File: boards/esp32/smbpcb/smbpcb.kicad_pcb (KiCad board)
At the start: 2 copper layers, 77.7 x 65.3 mm, 57 parts, among them IC1 MiCS-6814, J1 USB_B_Micro, J2 PMS7003, Q1 SUD08P06-155L, Q2 SS8050_NPN, Q3 SS8050_NPN, U1 MCP73831-2-OT, U2 TPS61200DRC, U3 ESP32-WROOM-32, U4 SSD1306, U5 BME680, U6 MH-Z19B

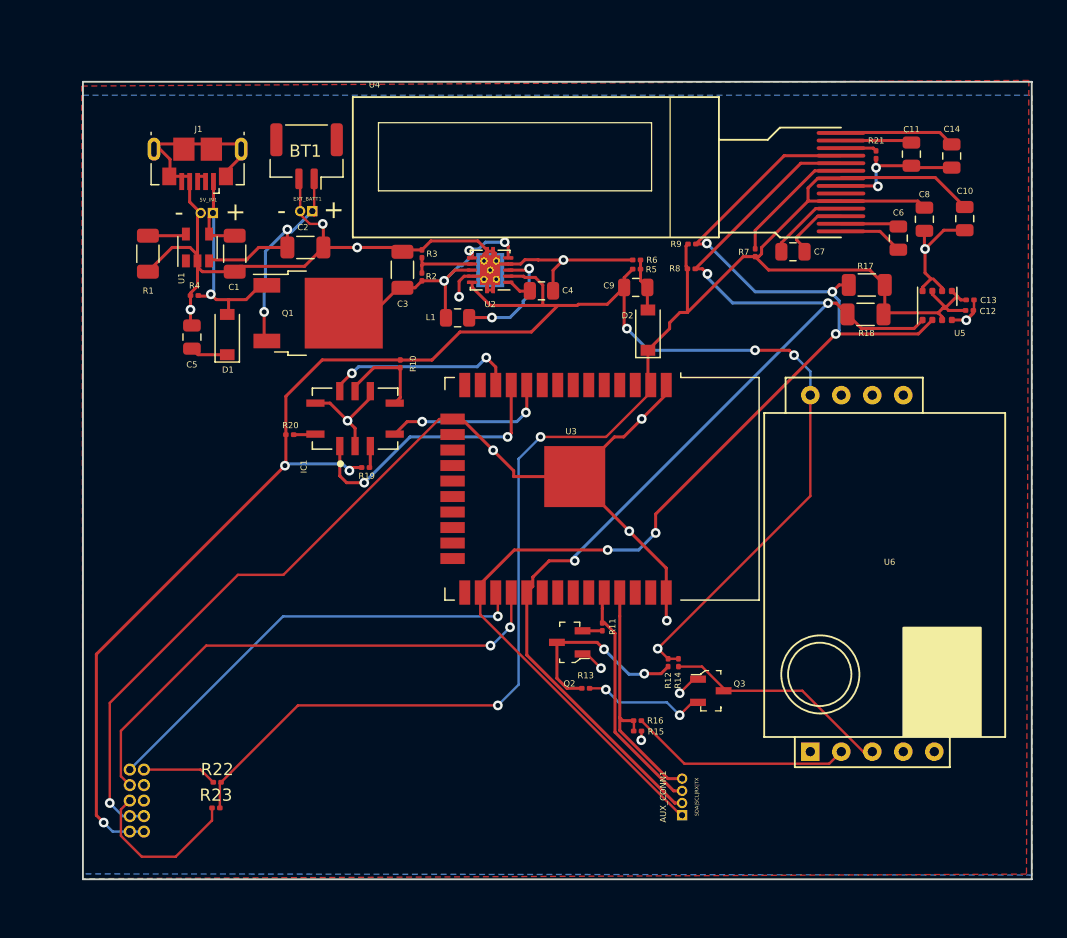
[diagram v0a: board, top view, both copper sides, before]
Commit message: more work'
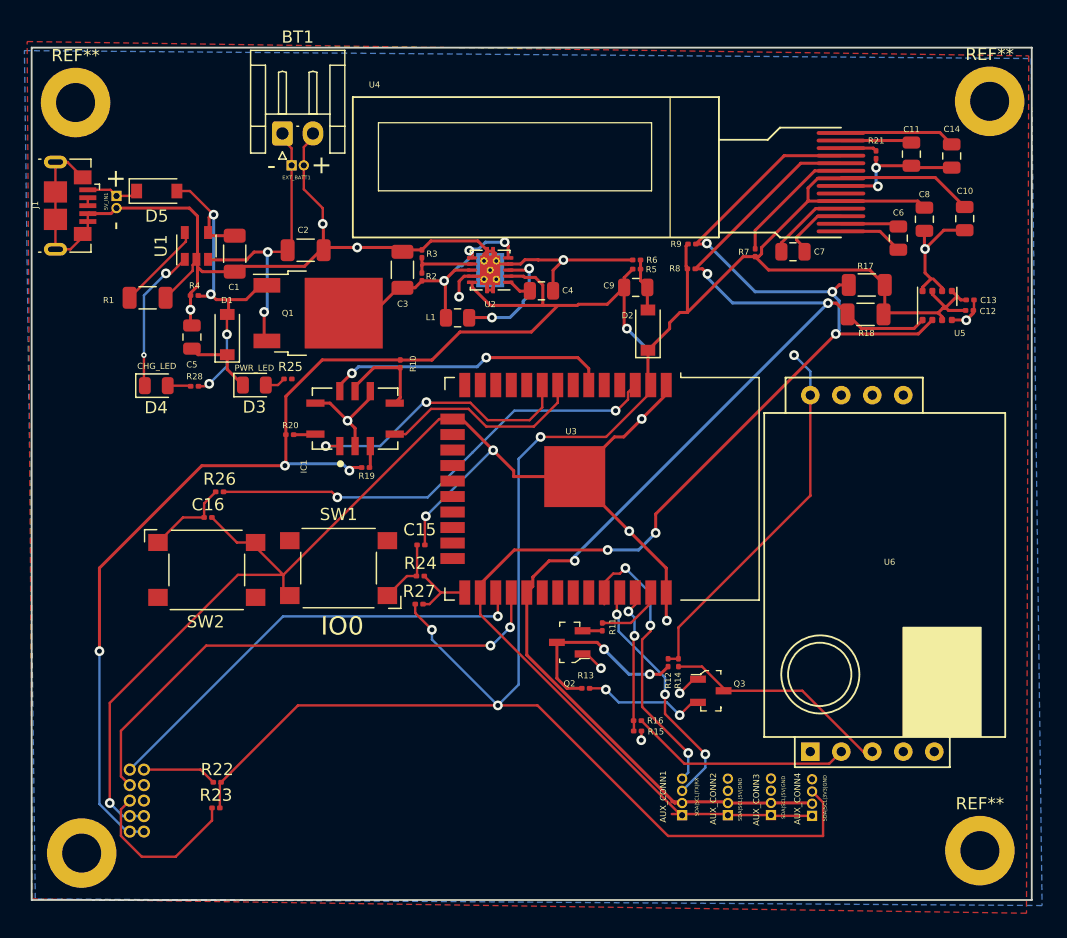
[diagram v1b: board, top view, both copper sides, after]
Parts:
- added ?: , , F.Cu at (74.1, 78.1)
- added AUX_CONN2: Conn_01x04_Female, Connector_PinHeader_1.00mm:PinHeader_1x04_P1.00mm_Vertical, F.Cu at (127.0, 75.0)
- added AUX_CONN3: Conn_01x04_Female, Connector_PinHeader_1.00mm:PinHeader_1x04_P1.00mm_Vertical, F.Cu at (130.6, 75.0)
- added AUX_CONN4: Conn_01x04_Female, Connector_PinHeader_1.00mm:PinHeader_1x04_P1.00mm_Vertical, F.Cu at (133.9, 75.0)
- added C15: 1nF, Capacitor_SMD:C_0201_0603Metric, F.Cu at (101.9, 52.9)
- added C16: 1nF, Capacitor_SMD:C_0201_0603Metric, F.Cu at (84.5, 50.6)
- added D3: PWR_LED, LED_SMD:LED_0805_2012Metric, F.Cu at (88.2, 39.8)
- added D4: PWR_LED, LED_SMD:LED_0805_2012Metric, F.Cu at (80.2, 39.8)
- added D5: D_Schottky, Diode_SMD:D_SOD-123, F.Cu at (80.2, 23.9)
- added R24: 470, Capacitor_SMD:C_0201_0603Metric, F.Cu at (101.8, 55.4)
- added R25: 2k, Capacitor_SMD:C_0201_0603Metric, F.Cu at (91.0, 39.2)
- added R26: 470, Capacitor_SMD:C_0201_0603Metric, F.Cu at (85.4, 48.5)
- added R27: 5.1k, Capacitor_SMD:C_0201_0603Metric, F.Cu at (101.8, 57.7)
- added R28: 470, Capacitor_SMD:C_0201_0603Metric, F.Cu at (83.3, 39.9)
- added REF**: MountingHole_3.2mm_M3_ISO7380_Pad, mountingholes:MountingHole_3.2mm_M3_ISO7380_Pad, F.Cu at (148.5, 16.5)
- added REF**: MountingHole_3.2mm_M3_ISO7380_Pad, mountingholes:MountingHole_3.2mm_M3_ISO7380_Pad, F.Cu at (147.7, 77.9)
- added REF**: MountingHole_3.2mm_M3_ISO7380_Pad, mountingholes:MountingHole_3.2mm_M3_ISO7380_Pad, F.Cu at (73.6, 16.6)
- added SW1: RESET, Button_Switch_SMD:SW_SPST_Omron_B3FS-101xP, F.Cu at (95.2, 54.8)
- added SW2: RESET, Button_Switch_SMD:SW_SPST_Omron_B3FS-101xP, F.Cu at (84.3, 54.9)
- BT1: footprint Connector_JST:JST_GH_SM02B-GHS-TB_1x02-1MP_P1.25mm_Horizontal -> Connector_JST:JST_EH_S2B-EH_1x02_P2.50mm_Horizontal
- R1: value 10k -> 2k
- moved J1 11.0 mm to (73.2, 25.1), turned to -90 degrees
- moved 5V_IN1 8.02 mm to (77.0, 24.2), turned to 0 degrees
- moved EXT_BATT1 4.12 mm to (91.3, 21.8), turned to 90 degrees
- moved R1 3.62 mm to (79.5, 32.6), turned to 0 degrees
- moved BT1 2.72 mm to (90.5, 19.1), turned to 0 degrees
- moved C2 0.22 mm to (92.5, 28.7)
- moved U1 0.15 mm to (83.5, 28.4)
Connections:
- AUX_CONN1 pad 3: ESP_RX0 -> ESP_TX0
- AUX_CONN1 pad 4: ESP_TX0 -> ESP_RX0
- C1 pad 1: Net-(5V_IN1-Pad1) -> Net-(C1-Pad1)
- D1 pad 2: Net-(5V_IN1-Pad1) -> Net-(C1-Pad1)
- J2 pad 7: ESP_RX1 -> ESP_RX2
- J2 pad 9: ESP_TX1 -> ESP_TX2
- Q1 pad 1: Net-(5V_IN1-Pad1) -> Net-(C1-Pad1)
- R11 pad 1: ESP_RX0 -> ESP_RX1
- R15 pad 2: ESP_TX0 -> ESP_TX1
- R16 pad 1: ESP_TX0 -> ESP_TX1
- R4 pad 1: Net-(5V_IN1-Pad1) -> Net-(C1-Pad1)
- U1 pad 1: unconnected-(U1-Pad1) -> Net-(D4-Pad1)
- U1 pad 4: Net-(5V_IN1-Pad1) -> Net-(C1-Pad1)
- U3 pad 10: NH3 -> unconnected-(U3-Pad10)
- U3 pad 11: NO2 -> unconnected-(U3-Pad11)
- U3 pad 12: CO -> unconnected-(U3-Pad12)
- U3 pad 25: unconnected-(U3-Pad25) -> IO0
- U3 pad 27: ESP_TX1 -> ESP_TX2
- U3 pad 28: ESP_RX1 -> ESP_RX2
- U3 pad 3: unconnected-(U3-Pad3) -> EN
- U3 pad 36: unconnected-(U3-Pad36) -> ESP_TX1
- U3 pad 37: unconnected-(U3-Pad37) -> ESP_RX1
- U3 pad 6: unconnected-(U3-Pad6) -> CO
- U3 pad 8: unconnected-(U3-Pad8) -> NH3
- U3 pad 9: unconnected-(U3-Pad9) -> NO2
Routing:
- net +3V3: track 140.5 -> 186.7 mm, vias 2 -> 3
- net ESP_RX2: track 0.00 -> 43.0 mm, vias 0 -> 2
- net EN: track 0.00 -> 38.1 mm, vias 0 -> 2
- net ESP_TX2: track 0.00 -> 37.4 mm, vias 0 -> 1
- net ESP_RX1: track 43.0 -> 5.72 mm, vias 2 -> 0
- net Net-(C1-Pad1): track 0.00 -> 29.1 mm, vias 0 -> 4
- net GND: track 209.3 -> 237.9 mm, vias 18 -> 19
- net ESP_TX1: track 37.4 -> 11.9 mm, vias 1 -> 2
- net Net-(5V_IN1-Pad1): track 20.6 -> 4.37 mm, vias 1 -> 0
- net Net-(D4-Pad1): track 0.00 -> 12.2 mm, vias 0 -> 2
- net SCL: track 95.4 -> 107.0 mm
- net SDA: track 106.1 -> 117.7 mm
- net +5V: track 147.8 -> 137.8 mm, vias 7 -> 5
- net CO: track 15.5 -> 23.1 mm
- net Net-(C16-Pad2): track 0.00 -> 7.12 mm
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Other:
- board size 77.7 x 65.3 mm -> 81.9 x 69.8 mm
- board text added: "CHG_LED"
- board text added: "IO0"
- board text added: "PWR_LED"
- board text added: "SDA|SCL|3V3|GND"
- board text added: "SDA|SCL|5V|GND"
- board text added: "SDA|SCL|TX|RX"
- board text removed: "SDA|SCL|RX|TX"
